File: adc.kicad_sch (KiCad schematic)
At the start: 43 parts, among them J1 Screw_Terminal_01x02, J2 Screw_Terminal_01x02, U1 Pico, U2 ADS8881CDGS, U3 LM4040DBZ-3, U4 OPA320AIDBVR, U5 THS4521ID, U6 OPA333xxD, U7 REF5045AD, U8 THS4281, U9 TPS7A49

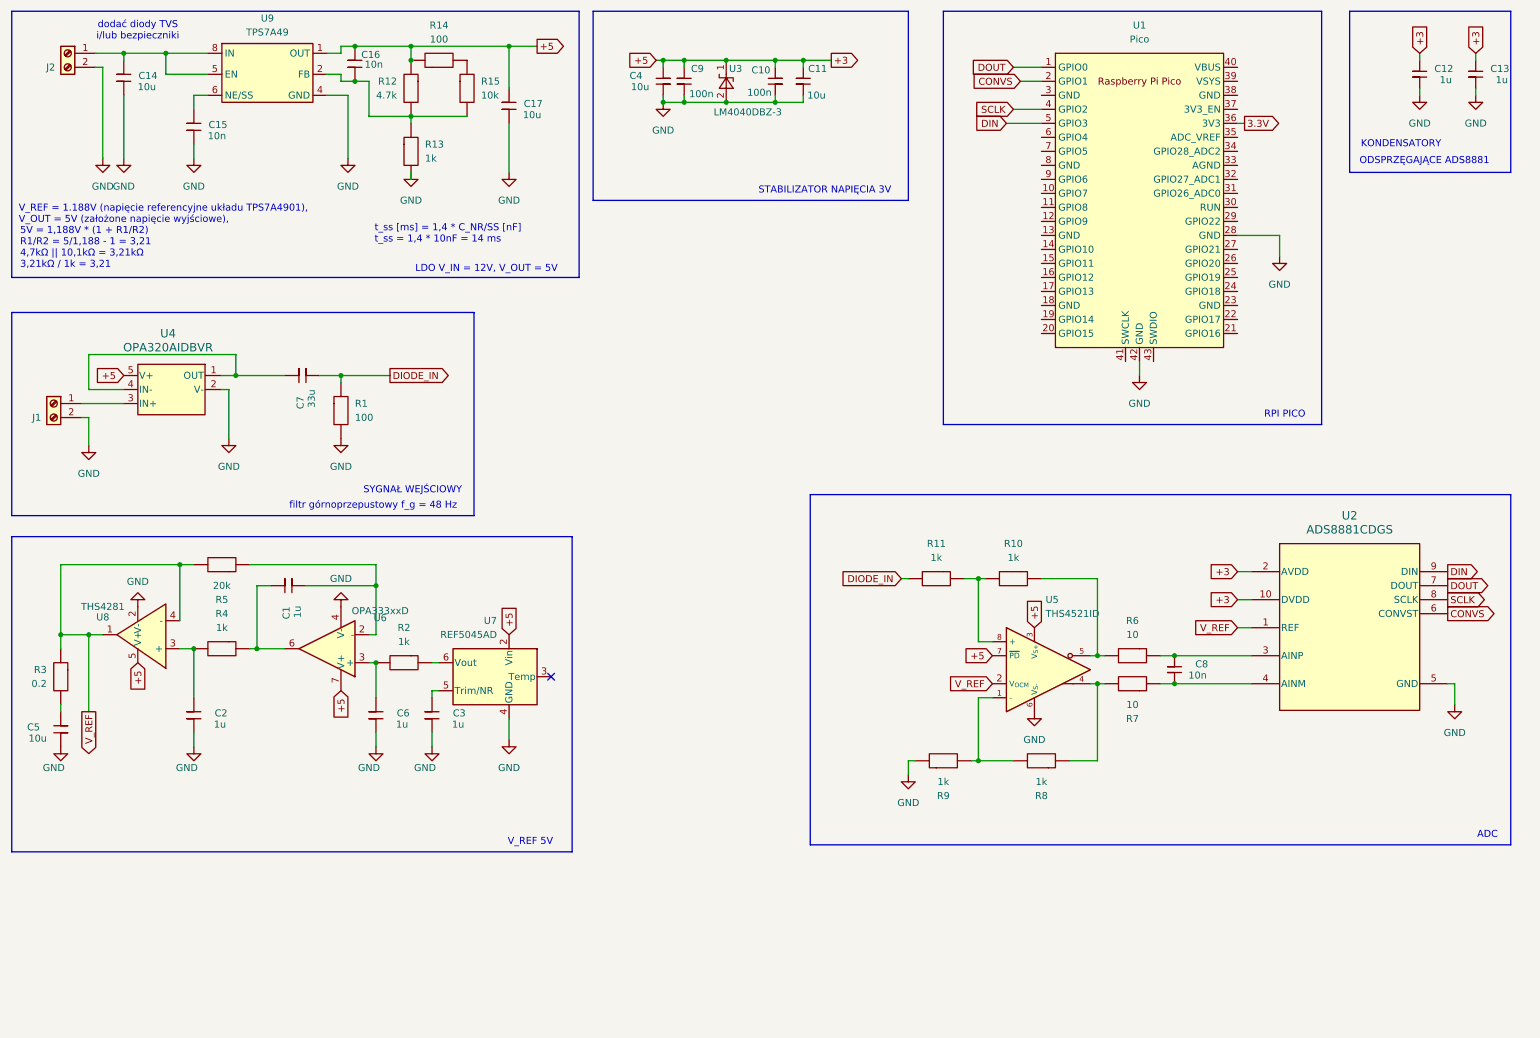
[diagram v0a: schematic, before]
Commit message: Add files via upload
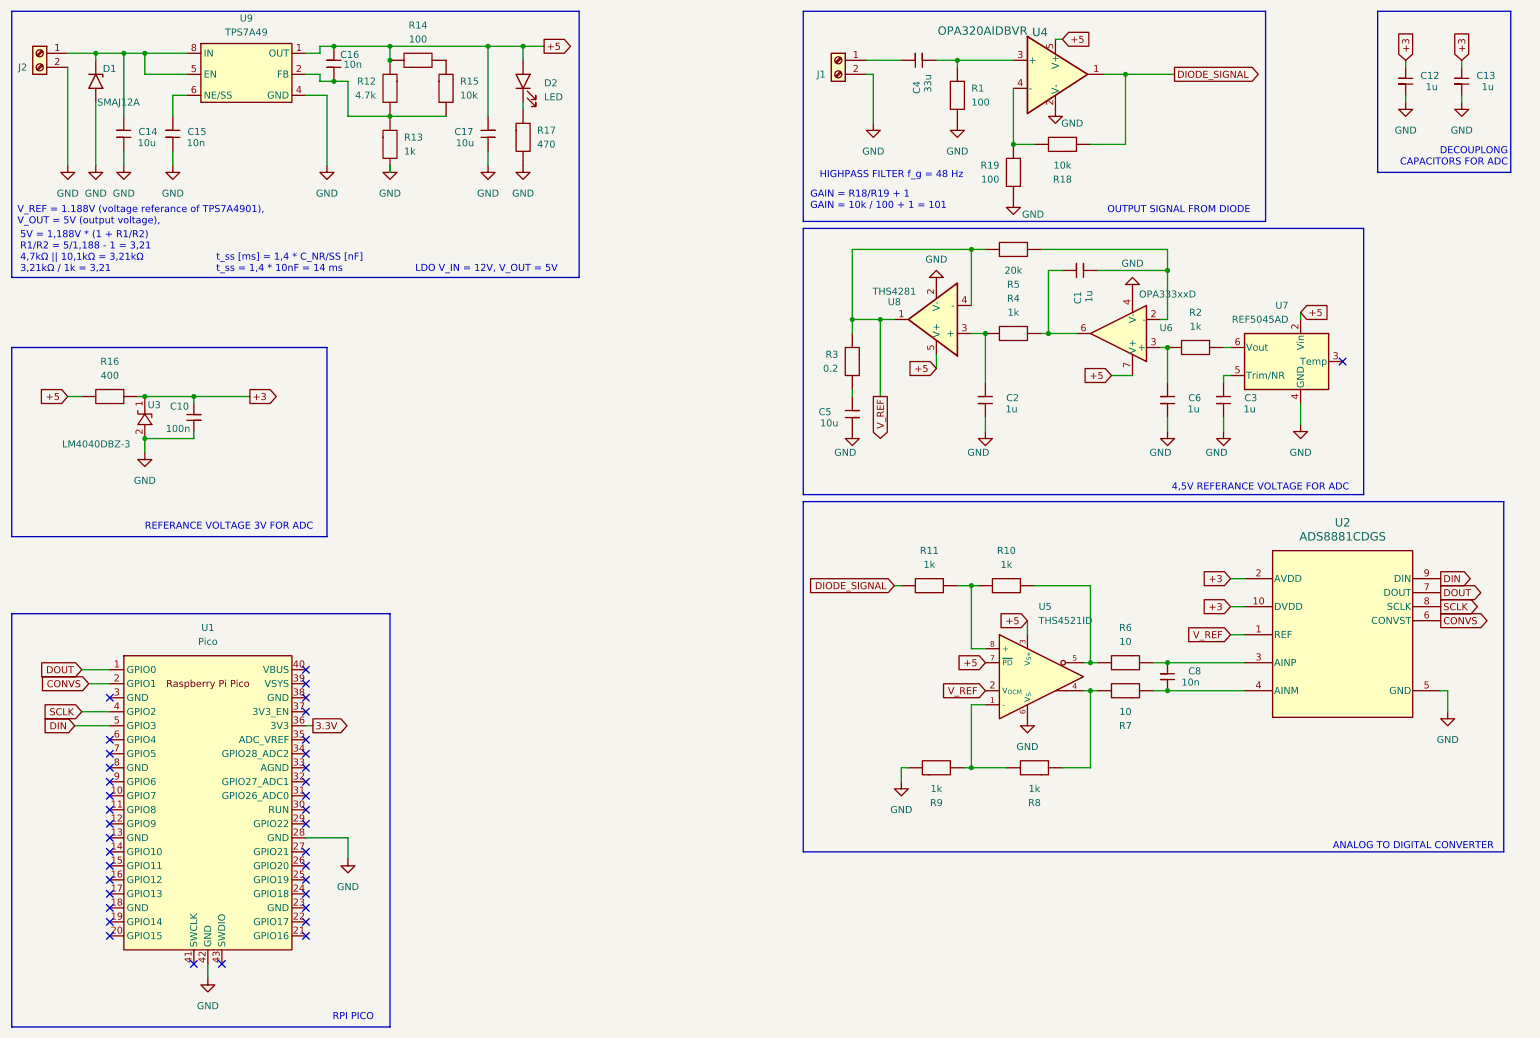
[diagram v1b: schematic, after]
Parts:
- removed C11: 10u, moja_biblioteka:cap_1206, symbol moja_biblioteka:cap_1206
- removed C7: 33u, moja_biblioteka:cap_1206, symbol moja_biblioteka:cap_1206
- removed C9: 100n, moja_biblioteka:cap_1206, symbol moja_biblioteka:cap_1206
- added D1: SMAJ12A, Diode_SMD:D_SMA, symbol Diode:SMAJ12A
- added D2: LED, moja_biblioteka:LED_SMD, symbol moja_biblioteka:LED_SMD
- added R16: 400, moja_biblioteka:res_1206, symbol moja_biblioteka:res_1206
- added R17: 470, moja_biblioteka:res_1206, symbol moja_biblioteka:res_1206
- added R18: 10k, moja_biblioteka:res_1206, symbol moja_biblioteka:res_1206
- added R19: 100, moja_biblioteka:res_1206, symbol moja_biblioteka:res_1206
- C4: value 10u -> 33u
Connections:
- net +3: now also R16.2; no longer C16.1, C17.1, C4.1, R12.1, R14.1, U4.5 (V+), U5.3 (V_{S+}), U5.7 (~{PD}), U6.7 (V+), U7.2 (Vin), U8.5 (V+), U9.1 (OUT)
- net GND: now also D1.2 (A2), R17.2, R19.2; no longer C4.2
- net at C14.1, J2.1 (Pin_1), U9.5 (EN)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: now also D1.1 (A1)
- net at U4.4 (-): now also R18.2, R19.1; no longer U4.1 (OUT)
- net at U4.3 (+): now also C4.2, R1.1; no longer J1.1 (Pin_1)
- net DIODE_IN renamed DIODE_SIGNAL
- net DIODE_SIGNAL: now also U4.1, R18.1; no longer R1.1
- new net: D2.1 (K), R17.1
- new net: C4.1, J1.1 (Pin_1)
- new net +5: C16.1, C17.1, D2.2 (A), R12.1, R14.1, R16.1, U4.5 (V+), U5.3 (V_{S+}), U5.7 (~{PD}), U6.7 (V+), U7.2 (Vin), U8.5 (V+), U9.1 (OUT)
- no-connect marks 1 -> 37
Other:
- note added: "4,5V REFERANCE VOLTAGE FOR ADC"
- note added: "ANALOG TO DIGITAL CONVERTER"
- note added: "DECOUPLONG CAPACITORS FOR ADC"
- note added: "GAIN = R18/R19 + 1 GAIN = 10k / 100 + 1 = 101"
- note added: "HIGHPASS FILTER f_g = 48 Hz"
- note added: "OUTPUT SIGNAL FROM DIODE"
- note added: "REFERANCE VOLTAGE 3V FOR ADC"
- note added: "V_REF = 1.188V (voltage referance of TPS7A4901), V_OUT = 5V (output voltage),"
- note removed: "ADC"
- note removed: "KONDENSATORY"
- note removed: "ODSPRZĘGAJĄCE ADS8881"
- note removed: "STABILIZATOR NAPIĘCIA 3V"
- note removed: "SYGNAŁ WEJŚCIOWY"
- note removed: "V_REF 5V"
- note removed: "V_REF = 1.188V (napięcie referencyjne układu TPS7A4901), V_OUT = 5V (założone napięcie wyjściowe),"
- note removed: "dodać diody TVS i/lub bezpieczniki"
- note removed: "filtr górnoprzepustowy f_g = 48 Hz"
- moved on the sheet: C1, C10, C12, C13, C14, C15, C16, C17, C2, C3, C5, C6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
